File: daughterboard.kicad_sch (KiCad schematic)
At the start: 0 parts

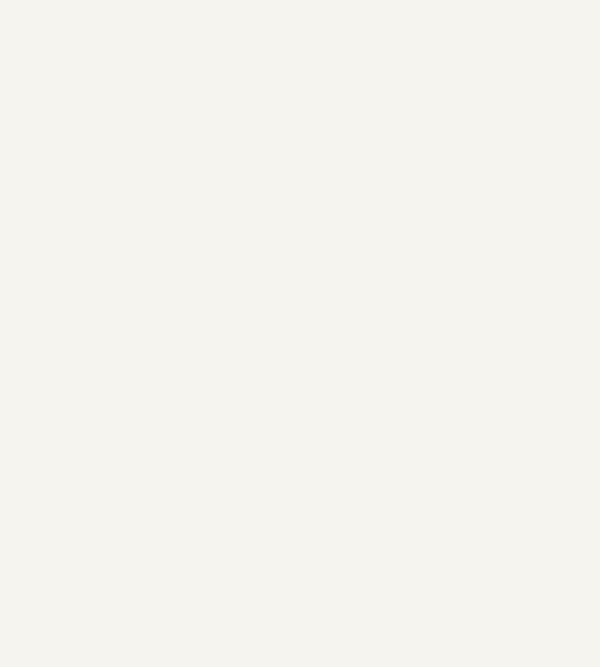
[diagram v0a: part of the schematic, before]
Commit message: Route power
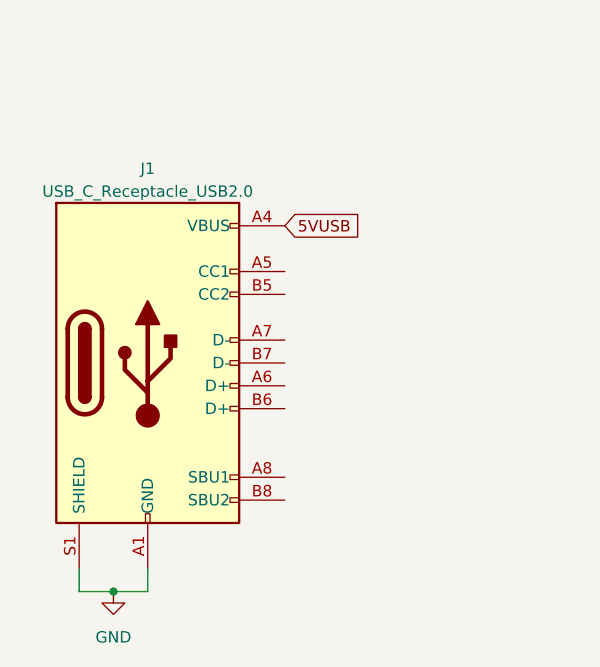
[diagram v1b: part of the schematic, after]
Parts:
- added J1: USB_C_Receptacle_USB2.0, Library:USB_C_GCT4105, symbol Connector:USB_C_Receptacle_USB2.0
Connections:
- new net 5VUSB: J1.A4 (VBUS), J1.A9 (VBUS), J1.B4 (VBUS), J1.B9 (VBUS)
- new net GND: J1.A1 (GND), J1.A12 (GND), J1.B1 (GND), J1.B12 (GND), J1.S1 (SHIELD)
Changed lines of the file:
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@@
 (kicad_sch (version 20230121) (generator eeschema)
   (paper "A4")
+  (junction (at 54.61 109.22) (diameter 0) (color 0 0 0 0)
+  )
+  (wire (pts (xy 54.61 109.22) (xy 58.42 109.22))
+    (stroke (width 0) (type default))
+  )
+  (wire (pts (xy 50.8 109.22) (xy 54.61 109.22))
+    (stroke (width 0) (type default))
+  )
+  (wire (pts (xy 58.42 109.22) (xy 58.42 106.68))
+    (stroke (width 0) (type default))
+  )
+  (wire (pts (xy 50.8 106.68) (xy 50.8 109.22))
+    (stroke (width 0) (type default))
+  )
+  (global_label "5VUSB" (shape input) (at 73.66 68.58 0) (fields_autoplaced)
+    (effects (font (size 1.27 1.27)) (justify left))
+    (property "Intersheetrefs" "${INTERSHEET_REFS}" (at 82.6739 68.58 0)
+      (effects (font (size 1.27 1.27)) (justify left) hide)
+    )
+  )
+  (symbol (lib_id "Connector:USB_C_Receptacle_USB2.0") (at 58.42 83.82 0) (unit 1)
+    (in_bom yes) (on_board yes) (dnp no) (fields_autoplaced)
+    (property "Reference" "J1" (at 58.42 62.23 0)
+      (effects (font (size 1.27 1.27)))
+    )
+    (property "Value" "USB_C_Receptacle_USB2.0" (at 58.42 64.77 0)
+      (effects (font (size 1.27 1.27)))
+    )
+    (property "Footprint" "Library:USB_C_GCT4105" (at 62.23 83.82 0)
+      (effects (font (size 1.27 1.27)) hide)
+    )
+    (property "Datasheet" "https://www.usb.org/sites/default/files/documents/usb_type-c.zip" (at 62.23 83.82 0)
+      (effects (font (size 1.27 1.27)) hide)
+    )
+    (pin "A1")
+    (pin "A12")
+    (pin "A4")
+    (pin "A5")
+    (pin "A6")
+    (pin "A7")
+    (pin "A8")
+    (pin "A9")
+    (pin "B1")
+    (pin "B12")
+    (pin "B4")
+    (pin "B5")
+    (pin "B6")
+    (pin "B7")
+    (pin "B8")
+    (pin "B9")
+    (pin "S1")
+    (instances
+      (project "daughterboard"
+        (path "/dce8b7ce-114c-4680-a1bd-14f36a94838a"
+          (reference "J1") (unit 1)
+        )
+      )
+    )
+  )
+  (symbol (lib_id "power:GND") (at 54.61 109.22 0) (unit 1)
+    (in_bom yes) (on_board yes) (dnp no) (fields_autoplaced)
+    (property "Reference" "#PWR026" (at 54.61 115.57 0)
+      (effects (font (size 1.27 1.27)) hide)
+    )
+    (property "Value" "GND" (at 54.61 114.3 0)
+      (effects (font (size 1.27 1.27)))
+    )
+    (property "Footprint" "" (at 54.61 109.22 0)
+      (effects (font (size 1.27 1.27)) hide)
+    )
+    (property "Datasheet" "" (at 54.61 109.22 0)
+      (effects (font (size 1.27 1.27)) hide)
+    )
+    (pin "1")
+    (instances
+      (project "daughterboard"
+        (path "/dce8b7ce-114c-4680-a1bd-14f36a94838a/233da297-15ca-4163-a51b-09f27dce3135"
+          (reference "#PWR026") (unit 1)
+        )
+        (path "/dce8b7ce-114c-4680-a1bd-14f36a94838a"
+          (reference "#PWR032") (unit 1)
+        )
+      )
+    )
+  )
   (sheet (at 123.19 48.26) (size 21.59 5.08) (fields_autoplaced)
     (stroke (width 0.1524) (type solid))
